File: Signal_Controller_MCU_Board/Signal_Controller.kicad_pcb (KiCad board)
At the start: 2 copper layers, 65 x 75 mm, 54 parts, among them J1 BARREL_JACK, J2 USB_OTG, J3 CONN_02X03, J4 CONN_01X03, J5 CONN_01X02, J6 CONN_01X02, J8 CONN_01X07, Q1 2N7002P,215, Q2 2N7002P,215, Q3 2N7002P,215, SW1 SW_Push, SW2 SW_Push, SW3 SW_Push, SW4 SW_Push, SW5 SW_Push, U1 AZ1117IH-5.0TRG1, U2 ATmega32U4, Y1 Crystal

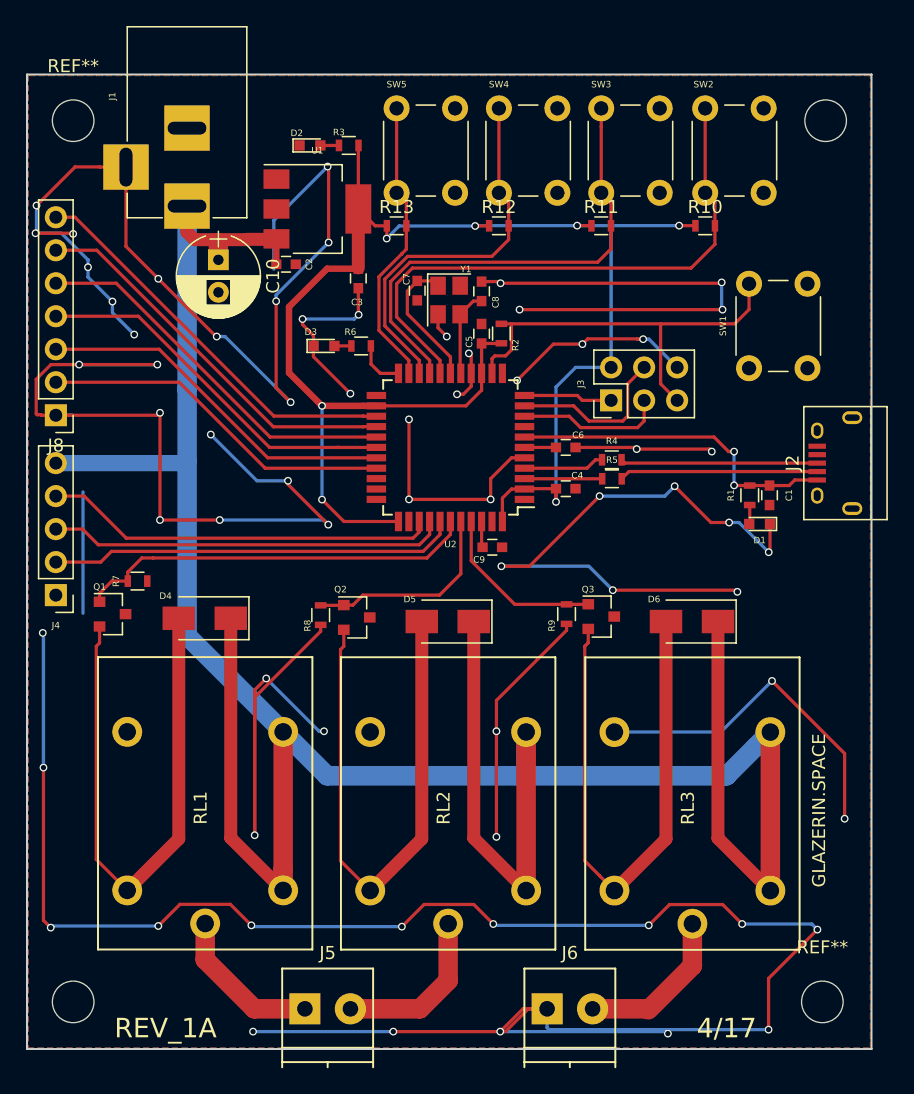
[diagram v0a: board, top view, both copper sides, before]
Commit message: I looked at it (minor tweaks)
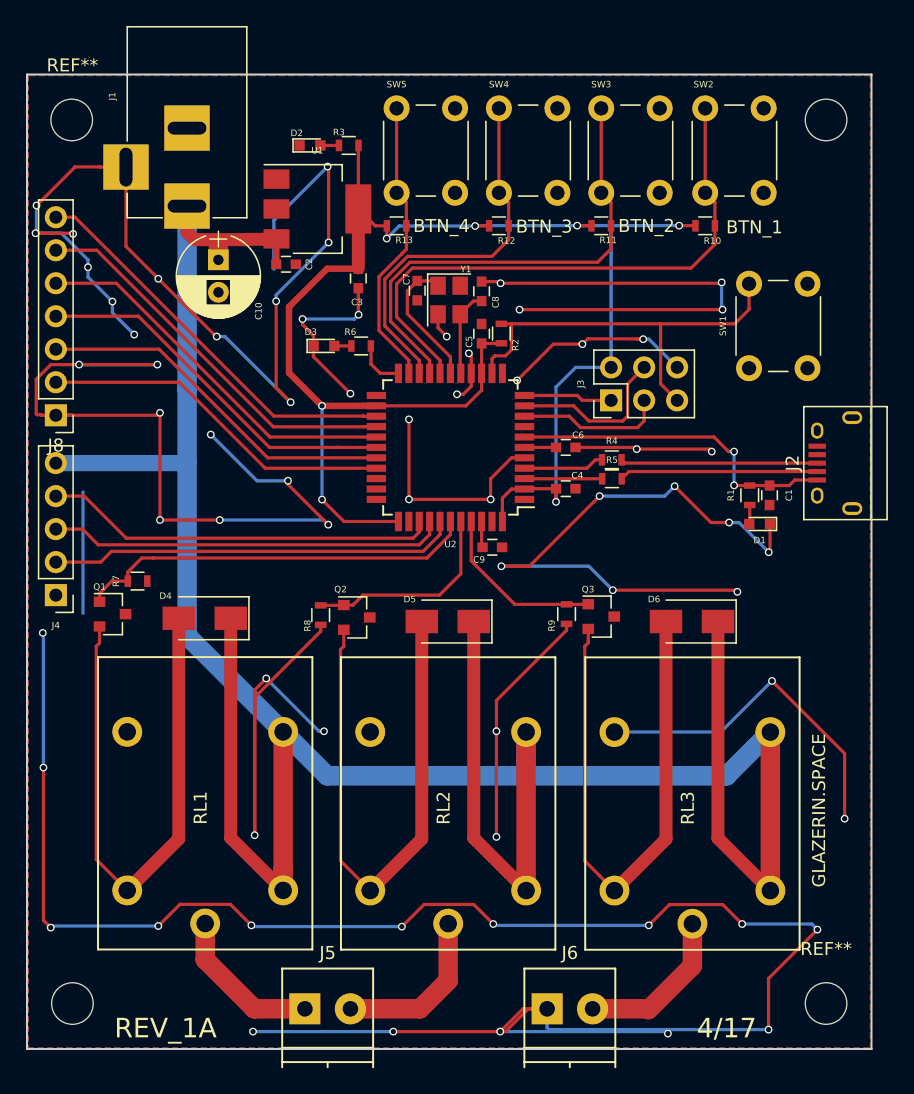
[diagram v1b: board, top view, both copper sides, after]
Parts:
- moved REF** 0.31 mm to (185.3, 129.0)
- moved ? 0.14 mm to (127.3, 129.0)
- moved REF** 0.08 mm to (127.3, 61.0)
- moved ? 0.06 mm to (185.3, 61.0)
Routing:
- net GND: track 496.9 -> 523.6 mm, vias 65 -> 67
- net (no net): track 36.0 -> 9.33 mm, vias 2 -> 0
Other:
- board text added: "BTN_1"
- board text added: "BTN_2"
- board text added: "BTN_3"
- board text added: "BTN_4"
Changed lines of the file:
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@@
   (general
     (links 140)
-    (no_connects 10)
-    (area -0.075001 -0.075001 65.075001 75.075001)
+    (no_connects 2)
+    (area 117.767857 53.433499 194.882143 136.5134)
     (thickness 1.6)
-    (drawings 7)
+    (drawings 11)
     (tracks 529)
     (zones 0)
@@
     (mod_text_size 1 1)
     (mod_text_width 0.15)
-    (pad_size 1.4 1.2)
-    (pad_drill 0)
+    (pad_size 3.2 3.2)
+    (pad_drill 3.2)
     (pad_to_mask_clearance 0.2)
     (aux_axis_origin 0 0)
     (visible_elements 7FFFFFFF)
     (pcbplotparams
-      (layerselection 0x00030_80000001)
-      (usegerberextensions false)
+      (layerselection 0x010ff_80000001)
+      (usegerberextensions true)
       (excludeedgelayer true)
       (linewidth 0.100000)
@@
       (outputformat 1)
       (mirror false)
-      (drillshape 1)
+      (drillshape 0)
       (scaleselection 1)
-      (outputdirectory ""))
+      (outputdirectory Gerbers/))
   )
   (net 0 "")
@@
   )
   (module Mounting_Holes:MountingHole_3.2mm_M3 (layer F.Cu)
-    (at 127.381 61.087)
+    (at 127.325 61.031)
     (descr "Mounting Hole 3.2mm, no annular, M3")
     (tags "mounting hole 3.2mm no annular m3")
@@
     (fp_circle (center 0 0) (end 3.2 0) (layer Cmts.User) (width 0.15))
     (fp_circle (center 0 0) (end 3.45 0) (layer F.CrtYd) (width 0.05))
-    (pad 1 np_thru_hole circle (at 0 0) (size 3.2 3.2) (drill 3.2) (layers *.Cu *.Mask))
+    (pad "" np_thru_hole circle (at -0.056 0) (size 3.2 3.2) (drill 3.2) (layers *.Cu *.Mask))
   )
   (module Mounting_Holes:MountingHole_3.2mm_M3 (layer F.Cu)
-    (at 185.293 61.087)
+    (at 185.325 61.031)
     (descr "Mounting Hole 3.2mm, no annular, M3")
     (tags "mounting hole 3.2mm no annular m3")
@@
   )
   (module Mounting_Holes:MountingHole_3.2mm_M3 (layer F.Cu)
-    (at 185.039 128.905)
+    (at 185.325 129.031)
     (descr "Mounting Hole 3.2mm, no annular, M3")
     (tags "mounting hole 3.2mm no annular m3")
@@
   )
   (module Mounting_Holes:MountingHole_3.2mm_M3 (layer F.Cu)
-    (at 127.381 128.905)
+    (at 127.325 129.031)
     (descr "Mounting Hole 3.2mm, no annular, M3")
     (tags "mounting hole 3.2mm no annular m3")
@@
       (effects (font (size 0.5 0.5) (thickness 0.125)))
     )
-    (fp_text value 1uF (at -1.8415 0 90) (layer F.Fab)
+    (fp_text value 1uF (at -0.7366 1.0668 180) (layer F.Fab)
       (effects (font (size 0.5 0.5) (thickness 0.125)))
     )
@@
     (tags "resistor 0603")
     (attr smd)
-    (fp_text reference R10 (at 0 -1.45) (layer F.SilkS)
-      (effects (font (size 1 1) (thickness 0.15)))
-    )
-    (fp_text value 10K (at 0 1.5) (layer F.Fab)
-      (effects (font (size 1 1) (thickness 0.15)))
+    (fp_text reference R10 (at 0.5588 1.1557) (layer F.SilkS)
+      (effects (font (size 0.5 0.5) (thickness 0.125)))
+    )
+    (fp_text value 10K (at -1.3462 -0.0127 90) (layer F.Fab)
+      (effects (font (size 0.5 0.5) (thickness 0.125)))
     )
     (fp_text user %R (at 0 0) (layer F.Fab)
@@
     (tags "resistor 0603")
     (attr smd)
-    (fp_text reference R11 (at 0 -1.45) (layer F.SilkS)
-      (effects (font (size 1 1) (thickness 0.15)))
-    )
-    (fp_text value 10K (at 0 1.5) (layer F.Fab)
-      (effects (font (size 1 1) (thickness 0.15)))
+    (fp_text reference R11 (at 0.5334 1.1049) (layer F.SilkS)
+      (effects (font (size 0.5 0.5) (thickness 0.125)))
+    )
+    (fp_text value 10K (at -1.27 0.0381 90) (layer F.Fab)
+      (effects (font (size 0.5 0.5) (thickness 0.125)))
     )
     (fp_text user %R (at 0 0) (layer F.Fab)
@@
     (tags "resistor 0603")
     (attr smd)
-    (fp_text reference R12 (at 0 -1.45) (layer F.SilkS)
-      (effects (font (size 1 1) (thickness 0.15)))
-    )
-    (fp_text value 10K (at 0 1.5) (layer F.Fab)
-      (effects (font (size 1 1) (thickness 0.15)))
+    (fp_text reference R12 (at 0.5842 1.1557) (layer F.SilkS)
+      (effects (font (size 0.5 0.5) (thickness 0.125)))
+    )
+    (fp_text value 10K (at -1.2954 0.0127 90) (layer F.Fab)
+      (effects (font (size 0.5 0.5) (thickness 0.125)))
     )
     (fp_text user %R (at 0 0) (layer F.Fab)
@@
     (tags "resistor 0603")
     (attr smd)
-    (fp_text reference R13 (at 0 -1.45) (layer F.SilkS)
-      (effects (font (size 1 1) (thickness 0.15)))
-    )
-    (fp_text value 10K (at 0 1.5) (layer F.Fab)
+    (fp_text reference R13 (at 0.5842 1.1049) (layer F.SilkS)
+      (effects (font (size 0.5 0.5) (thickness 0.125)))
+    )
+    (fp_text value 10K (at -1.3208 -0.0127 90) (layer F.Fab)
       (effects (font (size 0.5 0.5) (thickness 0.125)))
     )
@@
       (effects (font (size 0.5 0.5) (thickness 0.125)))
     )
-    (fp_text value AZ1117IH-5.0TRG1 (at -1.4605 4.064) (layer F.Fab)
+    (fp_text value AZ1117IH-5.0TRG1 (at 0.3302 -3.8989) (layer F.Fab)
       (effects (font (size 0.5 0.5) (thickness 0.125)))
     )
@@
       (effects (font (size 0.5 0.5) (thickness 0.125)))
     )
-    (fp_text value SW_Push (at 3.75 6.7 90) (layer F.Fab)
+    (fp_text value SW_Push (at 3.2893 2.2352 90) (layer F.Fab)
       (effects (font (size 1 1) (thickness 0.15)))
     )
@@
       (effects (font (size 0.5 0.5) (thickness 0.125)))
     )
-    (fp_text value SW_Push (at 3.75 6.7 90) (layer F.Fab)
+    (fp_text value SW_Push (at 3.1369 2.2352 90) (layer F.Fab)
       (effects (font (size 1 1) (thickness 0.15)))
     )
@@
     (descr "CP, Radial series, Radial, pin pitch=2.50mm, , diameter=6.3mm, Electrolytic Capacitor")
     (tags "CP Radial series Radial pin pitch 2.50mm  diameter 6.3mm Electrolytic Capacitor")
-    (fp_text reference C10 (at 1.25 -4.21 270) (layer F.SilkS)
-      (effects (font (size 1 1) (thickness 0.15)))
+    (fp_text reference C10 (at 3.9478 -3.0988 270) (layer F.SilkS)
+      (effects (font (size 0.5 0.5) (thickness 0.125)))
     )
     (fp_text value CP1 (at 1.25 4.21 270) (layer F.Fab)
@@
     )
   )
+  (gr_text BTN_4 (at 155.7274 69.1896) (layer F.SilkS)
+    (effects (font (size 1 1) (thickness 0.25)))
+  )
+  (gr_text BTN_3 (at 163.6268 69.2404) (layer F.SilkS)
+    (effects (font (size 1 1) (thickness 0.25)))
+  )
+  (gr_text BTN_2 (at 171.5008 69.1896) (layer F.SilkS)
+    (effects (font (size 1 1) (thickness 0.25)))
+  )
+  (gr_text BTN_1 (at 179.8066 69.2912) (layer F.SilkS)
+    (effects (font (size 1 1) (thickness 0.25)))
+  )
   (gr_text GLAZERIN.SPACE (at 184.785 114.173 90) (layer F.SilkS)
     (effects (font (size 1 1) (thickness 0.25)))
@@
   (gr_line (start 123.825 57.531) (end 123.825 132.531) (angle 90) (layer Edge.Cuts) (width 0.15))
   (segment (start 128.143 89.662) (end 128.143 98.9965) (width 0.25) (layer B.Cu) (net 0))
-  (segment (start 181.1655 104.2035) (end 186.7535 109.7915) (width 0.25) (layer F.Cu) (net 0))
-  (segment (start 186.7535 109.7915) (end 186.7535 114.808) (width 0.25) (layer F.Cu) (net 0))
-  (via (at 186.7535 114.808) (size 0.6) (drill 0.4) (layers F.Cu B.Cu) (net 0))
-  (segment (start 169.037 108.1405) (end 177.2285 108.1405) (width 0.25) (layer B.Cu) (net 0))
-  (segment (start 177.2285 108.1405) (end 181.1655 104.2035) (width 0.25) (layer B.Cu) (net 0))
-  (via (at 181.1655 104.2035) (size 0.6) (drill 0.4) (layers F.Cu B.Cu) (net 0))
   (segment (start 162.1155 85.433) (end 176.702736 85.433) (width 0.25) (layer F.Cu) (net 1))
   (segment (start 176.702736 85.433) (end 177.820236 86.5505) (width 0.25) (layer F.Cu) (net 1))
@@
   (segment (start 180.975 89.166) (end 182.487 89.166) (width 0.25) (layer F.Cu) (net 1))
   (segment (start 179.451 89.166) (end 180.975 89.166) (width 0.25) (layer F.Cu) (net 1))
+  (segment (start 181.1655 104.2035) (end 186.7535 109.7915) (width 0.25) (layer F.Cu) (net 2))
+  (segment (start 186.7535 109.7915) (end 186.7535 114.808) (width 0.25) (layer F.Cu) (net 2))
+  (via (at 186.7535 114.808) (size 0.6) (drill 0.4) (layers F.Cu B.Cu) (net 2))
+  (segment (start 169.037 108.1405) (end 177.2285 108.1405) (width 0.25) (layer B.Cu) (net 2))
+  (segment (start 177.2285 108.1405) (end 181.1655 104.2035) (width 0.25) (layer B.Cu) (net 2))
+  (via (at 181.1655 104.2035) (size 0.6) (drill 0.4) (layers F.Cu B.Cu) (net 2))
   (segment (start 146.9644 64.6176) (end 142.8242 68.7578) (width 0.25) (layer B.Cu) (net 2))
   (segment (start 142.8242 68.7578) (end 142.8242 72.517) (width 0.25) (layer B.Cu) (net 2))
